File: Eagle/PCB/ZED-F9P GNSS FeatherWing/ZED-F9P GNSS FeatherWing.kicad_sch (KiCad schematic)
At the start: 43 parts, among them CON1 MICROBUILDER_USBFCI_10103594_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, J1 Coupler_v2_Coupler_v2-rescue_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, Q1 DMG2305, U1 ZED-F9P_ZED-F9P, U2 SPX3819-3.3, X1 SMA-142-0711-821/826

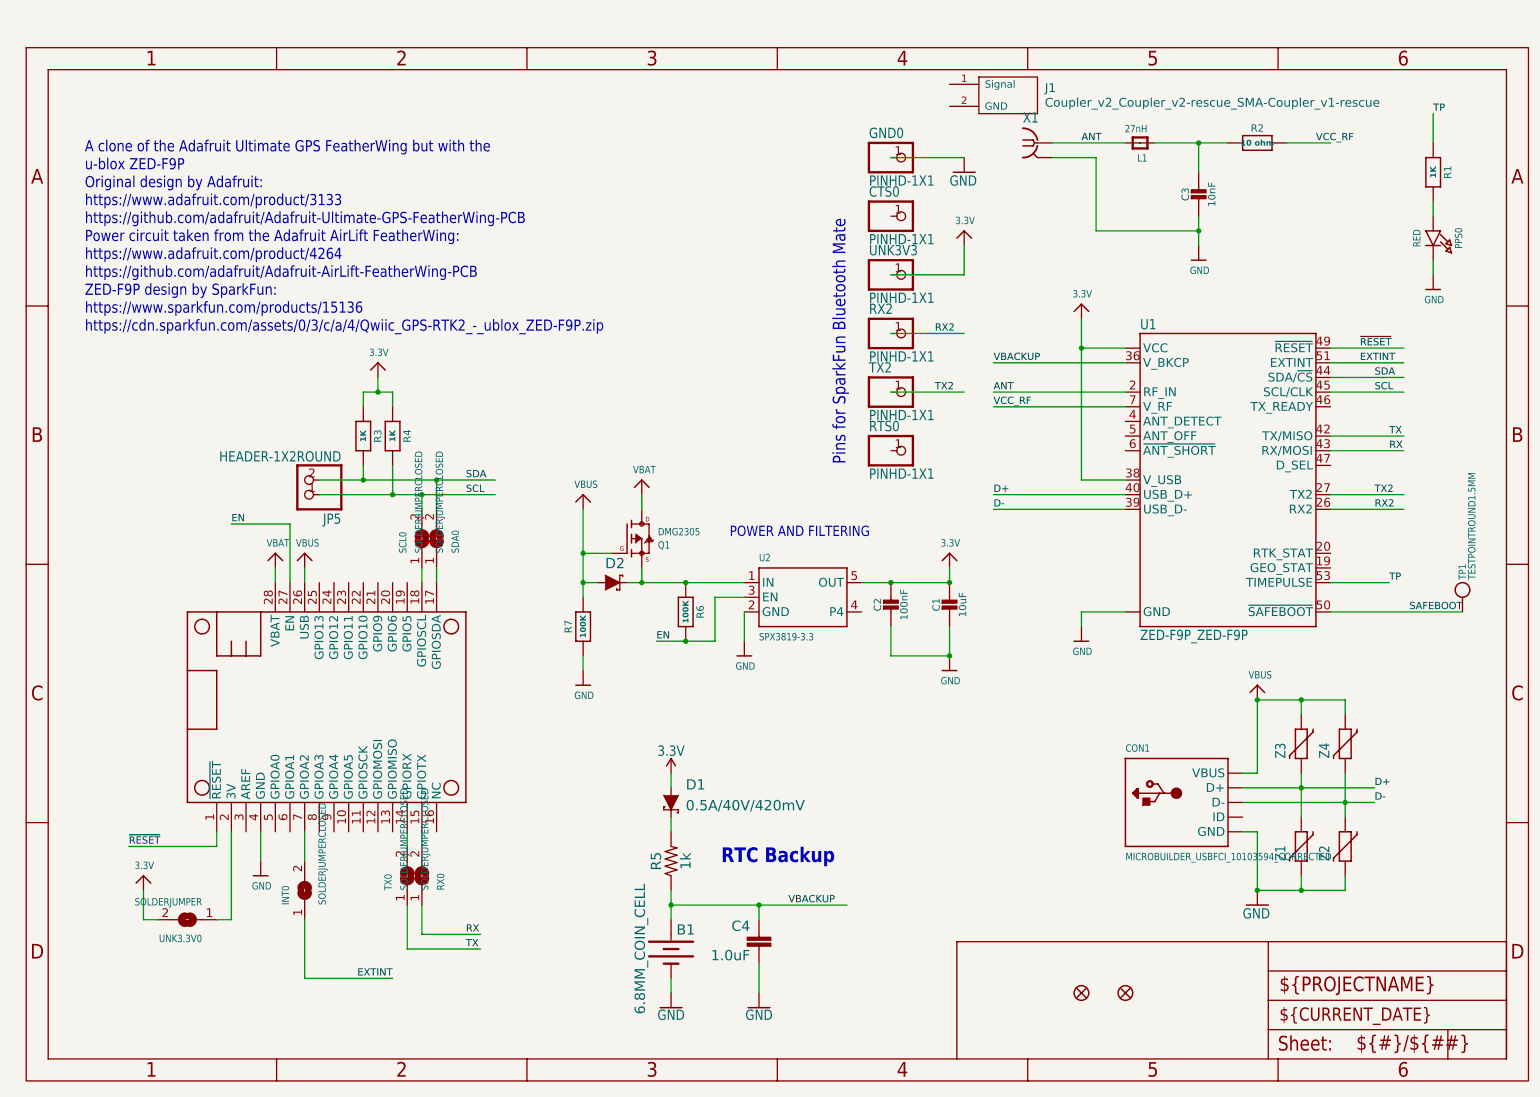
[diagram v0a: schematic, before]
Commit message: V2 Release
Released to fab.
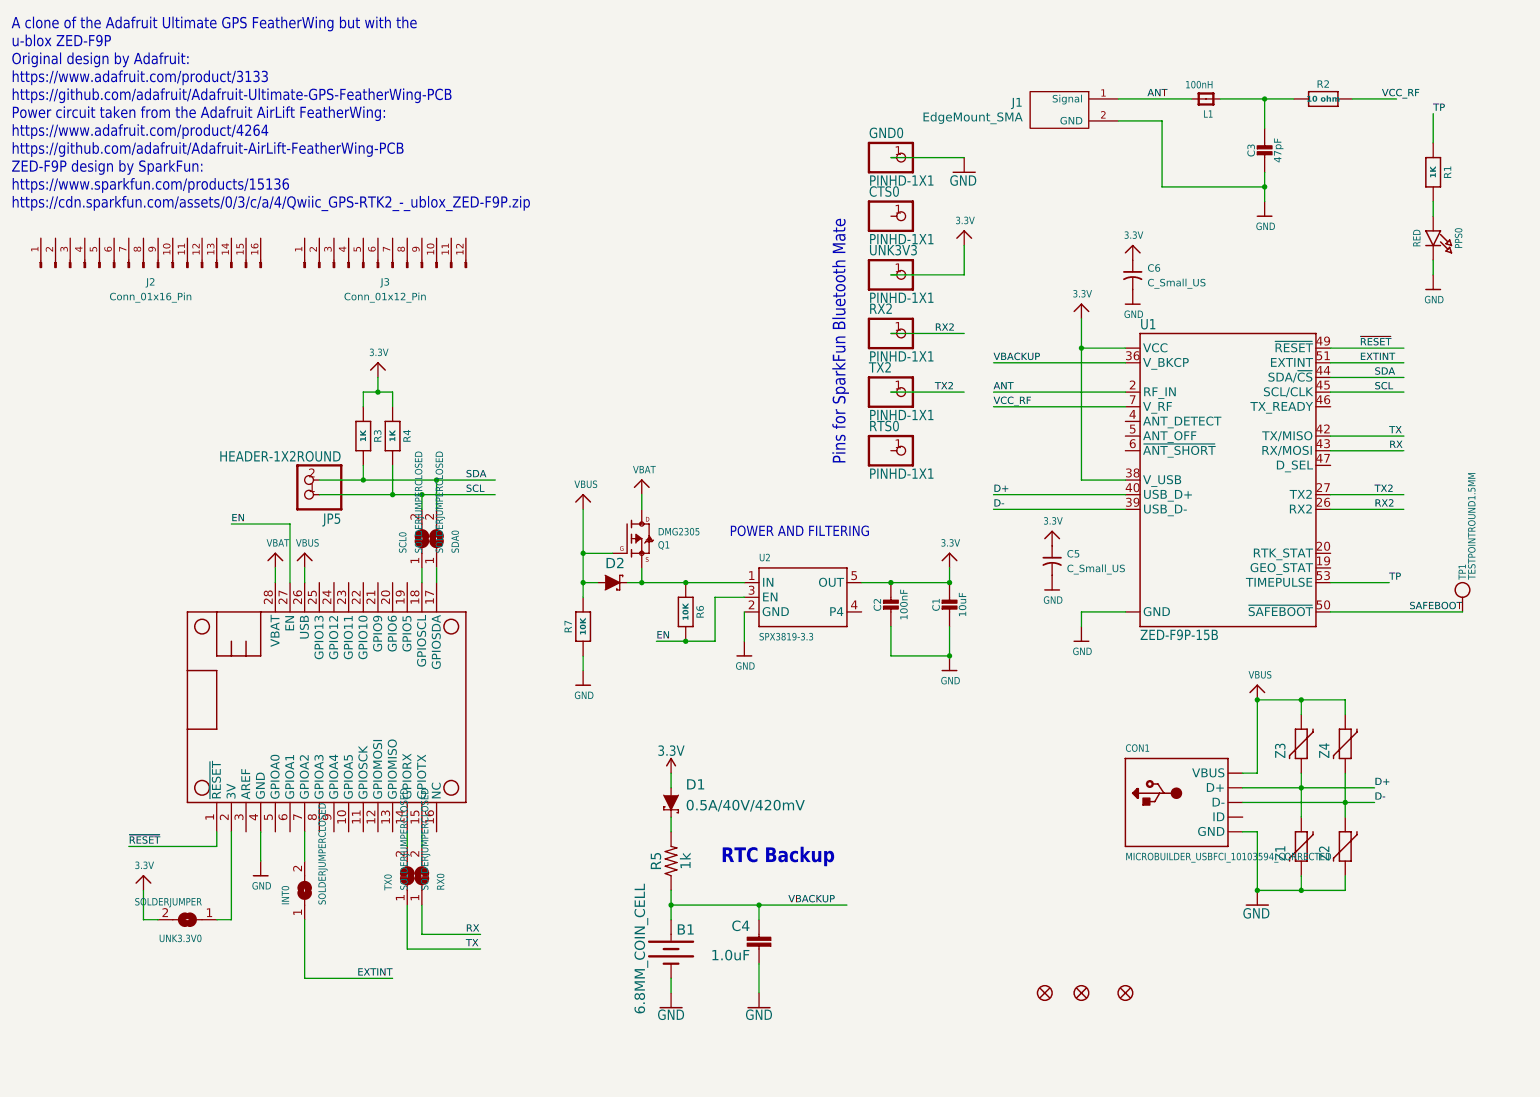
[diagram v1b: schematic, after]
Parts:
- removed X1: SMA-142-0711-821/826, ZED-F9P GNSS FeatherWing:J502-ND-142-0711-821_826_133, symbol ZED-F9P GNSS FeatherWing-eagle-import:SMA-142-0711-821/826
- added C5, C6: C_Small_US, Capacitor_SMD:C_0402_1005Metric, symbol Device:C_Small_US
- added FID3: FIDUCIAL{dblquote}{dblquote}, Fiducial:Fiducial_0.5mm_Mask1mm, symbol ZED-F9P GNSS FeatherWing-eagle-import:FIDUCIAL{dblquote}{dblquote}
- added J2: Conn_01x16_Pin, symbol Connector:Conn_01x16_Pin
- added J3: Conn_01x12_Pin, symbol Connector:Conn_01x12_Pin
- B1: Digikey PN (none) -> 728-1057-ND; Manu (none) -> Seiko Instruments; Manu PN (none) -> Seiko Instruments
- C1: Digikey PN (none) -> 1276-1298-1-ND; Manu (none) -> Samsung Electro-Mechanics; Manu PN (none) -> CL21A106MQFNNNE; Voltage (none) -> 6.3V
- C2: Digikey PN (none) -> 1276-2442-1-ND; Manu (none) -> Samsung Electro-Mechanics; Manu PN (none) -> CL21B104KACNFNC; Voltage (none) -> 25V
- C3: value 10nF -> 47pF; footprint ZED-F9P GNSS FeatherWing:0805-NO -> Capacitor_SMD:C_0402_1005Metric; Digikey PN (none) -> 490-14446-1-ND; Manu PN (none) -> GJM1555C1H470JB01D
- C4: Digikey PN (none) -> 1276-1945-1-ND; Manu (none) -> Samsung Electro-Mechanics; Manu PN (none) -> CL10B105KP8NFNC; Voltage (none) -> 10V
- CON1: Digikey PN (none) -> 609-4050-1-ND; Manu (none) -> Amphenol ICC (FCI); Manu PN (none) -> 10103594-0001LF
- CTS0, GND0, JP5, MS1, RTS0, RX2, TP1, TX2, UNK3V3: now left out of the parts list
- D1, D2: Digikey PN (none) -> 1801-BAT201M3RRGCT-ND; Manu (none) -> Taiwan Semiconductor Corporation; Manu PN (none) -> BAT201M3 RRG
- FID1, FID2: footprint ZED-F9P GNSS FeatherWing:FIDUCIAL_1MM -> Fiducial:Fiducial_0.5mm_Mask1mm; now left out of the parts list
- INT0, RX0, SCL0, SDA0, TX0: footprint ZED-F9P GNSS FeatherWing:SOLDERJUMPER_CLOSEDWIRE -> Jumper:SolderJumper-2_P1.3mm_Bridged_RoundedPad1.0x1.5mm; now left out of the parts list
- J1: value Coupler_v2_Coupler_v2-rescue_SMA-Coupler_v1-rescue -> EdgeMount_SMA; footprint Coupler_v1:SMA_Molex_732511150_v3 -> Coupler_v1:SMA_Molex_0732512120; Digikey PN (none) -> WM5536-ND; Manu (none) -> Molex; Manu PN (none) -> 0732512120
- L1: value 27nH -> 100nH; footprint ZED-F9P GNSS FeatherWing:0805-NO -> Inductor_SMD:L_0603_1608Metric; Digikey PN (none) -> 490-15766-1-ND; Manu PN (none) -> LQW18ANR10G8ZD
- PPS0: Digikey PN (none) -> 732-4984-1-ND; Manu (none) -> Würth Elektronik; Manu PN (none) -> 150080RS75000
- Q1: Digikey PN (none) -> FDN340PCT-ND; Manu (none) -> onsemi; Manu PN (none) -> FDN340P
- R1, R3, R4, R5: Digikey PN (none) -> 13-RT0603FRE131KLCT-ND; Manu (none) -> YAGEO; Manu PN (none) -> RT0603FRE131KL
- R2: footprint ZED-F9P GNSS FeatherWing:0805-NO -> Resistor_SMD:R_0402_1005Metric; Digikey PN (none) -> CR0402-JW-100GLFCT-ND; Manu (none) -> Bourns Inc.; Manu PN (none) -> CR0402-JW-100GLF
- R6, R7: value 100K -> 10K; Digikey PN (none) -> RNCP0603FTD10K0CT-ND; Manu (none) -> Stackpole Electronics Inc; Manu PN (none) -> RNCP0603FTD10K0
- U1: value ZED-F9P_ZED-F9P -> ZED-F9P-15B; Digikey PN (none) -> 672-ZED-F9P-15BCT-ND; Manu (none) -> u-blox; Manu PN (none) -> ZED-F9P-15B
- U2: Digikey PN (none) -> 1016-1873-1-ND; Manu (none) -> MaxLinear, Inc.; Manu PN (none) -> SPX3819M5-L-3-3/TR
- UNK3.3V0: footprint ZED-F9P GNSS FeatherWing:SOLDERJUMPER_ARROW_NOPASTE -> Jumper:SolderJumper-2_P1.3mm_Open_RoundedPad1.0x1.5mm; now left out of the parts list
- Z1, Z2, Z3, Z4: Digikey PN (none) -> CG0603MLC-05ECT-ND; Manu (none) -> Bourns Inc.; Manu PN (none) -> CG0603MLC-05E
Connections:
- net 3.3V: now also C5.1, C6.1
- net ANT: now also J1.1 (Signal)
- net GND: now also J1.2 (GND), C5.2, C6.2
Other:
- moved on the sheet: C3, J1, L1, R2
